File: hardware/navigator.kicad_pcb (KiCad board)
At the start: 4 copper layers, 65 x 56.5 mm, 45 parts, among them J1 BLDC-1, J10 GPIO, J2 BLDC-1, J3 BLDC-1, J4 BLDC-1, J5 BLDC-1, J6 BLDC-1, J7 Conn_01x02_Pin, J8 USB_C_Receptacle_USB2.0_16P, J9 Conn_01x04_Pin, SW1 SW_SPST, SW2 SW_SPST, U1 AP2112K-3.3, U2 LM2576-5.0, U3 ESP32-S3-MINI-1U, U4 INA226

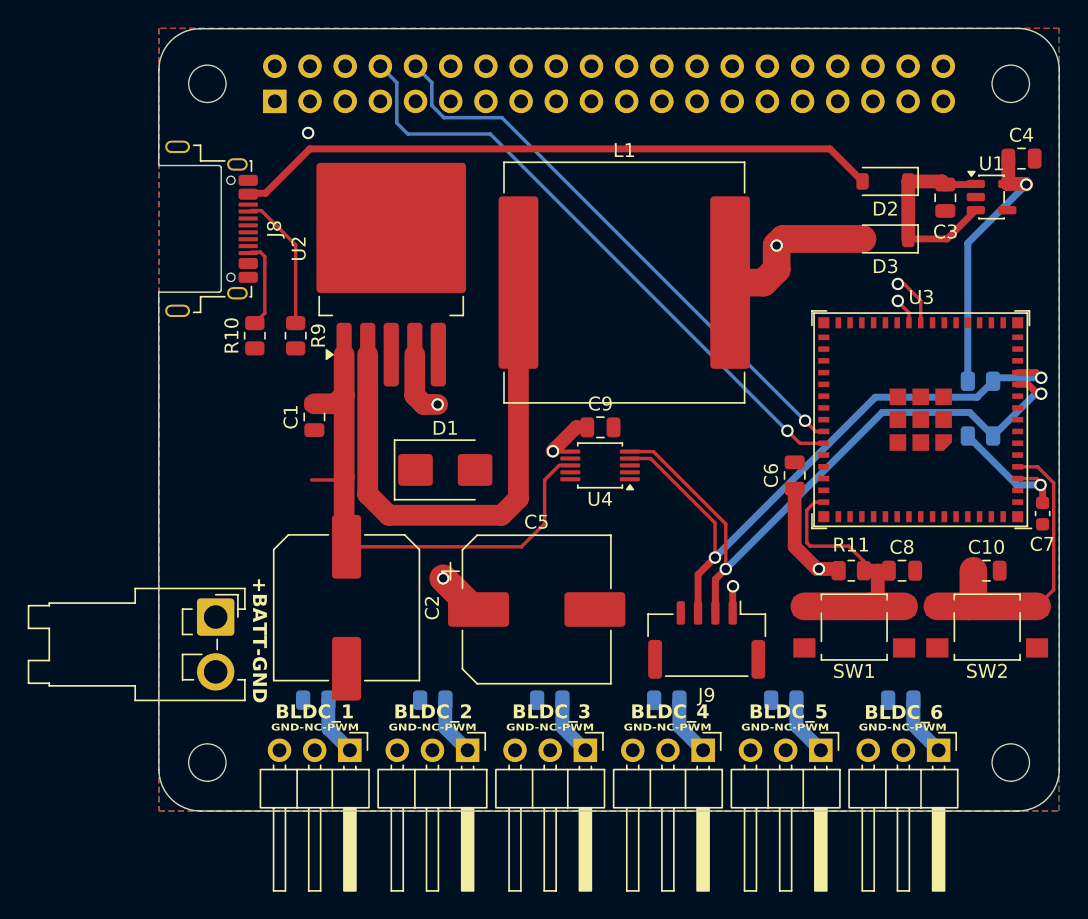
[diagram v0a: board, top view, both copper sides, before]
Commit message: feat: update navigator hardware to revision 002
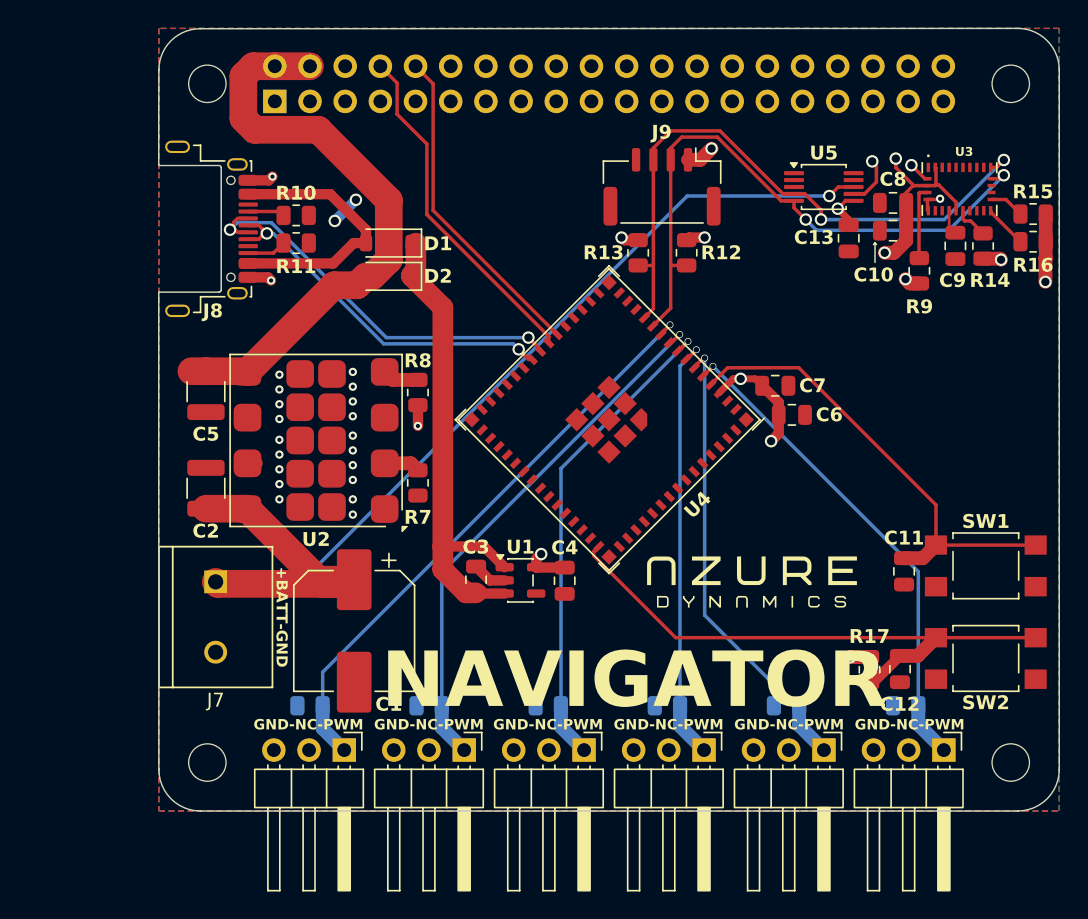
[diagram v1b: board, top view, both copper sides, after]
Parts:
- removed D3: D_Schottky, Diode_SMD:D_SOD-123
- removed L1: 100uH, Inductor_SMD:L_Vishay_IHLP-6767
- removed the U4 at (131.8, 75.0)
- added C11: 0.1uF, Capacitor_SMD:C_0805_2012Metric, F.Cu at (153.8, 82.7)
- added C12: 1uF, Capacitor_SMD:C_0805_2012Metric, F.Cu at (153.5, 89.8)
- added C13: 0.1uF, Capacitor_SMD:C_0805_2012Metric, F.Cu at (149.8, 58.6)
- added G***: LOGO, logo:logo, F.Cu at (142.8, 83.4)
- added R12: 2k2, Resistor_SMD:R_0805_2012Metric, F.Cu at (138.1, 59.7)
- added R13: 2k2, Resistor_SMD:R_0805_2012Metric, F.Cu at (134.6, 59.7)
- added R14: 10k, Resistor_SMD:R_0805_2012Metric, F.Cu at (159.5, 59.2)
- added R15: 10k, Resistor_SMD:R_0805_2012Metric, F.Cu at (163.1, 56.9)
- added R16: 10k, Resistor_SMD:R_0805_2012Metric, F.Cu at (163.1, 58.9)
- added R17: 10k, Resistor_SMD:R_0805_2012Metric, F.Cu at (151.3, 89.8)
- added U3: BNO086, BNO086:BNO086, F.Cu at (157.8, 55.1)
- added U5: INA226, Package_SO:TSSOP-10_3x3mm_P0.5mm, F.Cu at (148.0, 55.0)
- C1: value 0.1uF -> 100uF; footprint Capacitor_SMD:C_0805_2012Metric -> Capacitor_SMD:CP_Elec_8x10.5
- C2: value 330uF -> 10uF; footprint Capacitor_SMD:C_Elec_10x10.2 -> Capacitor_SMD:C_1210_3225Metric
- C5: value 1000uF -> 47uF; footprint Capacitor_SMD:CP_Elec_10x10.5 -> Capacitor_SMD:C_1210_3225Metric
- C7: footprint Capacitor_SMD:C_0603_1608Metric -> Capacitor_SMD:C_0805_2012Metric
- C8: value 1uF -> 0.1uF
- D1: value Schottky -> D_Schottky; footprint Diode_SMD:D_SMB -> Diode_SMD:D_SOD-123
- J7: footprint Connector_JST:JST_VH_S2P-VH_1x02_P3.96mm_Horizontal -> 282837-2:282837-2
- R11: value 10k -> 5k1
- R7: value 2k2 -> 100k; moved to F.Cu
- R8: value 2k2 -> 14k3; moved to F.Cu
- R9: value 5k1 -> 10k
- U2: value LM2576-5.0 -> MPM3550EGLE; footprint Package_TO_SOT_SMD:TO-263-5_TabPin3 -> Package_LGA:MPS_LGA-18-10EP_12x12mm_P3.3mm
- moved R11 46.5 mm to (109.9, 59.0), turned to 180 degrees
- moved R9 45.3 mm to (154.9, 61.0), turned to 90 degrees
- moved C4 44.9 mm to (129.3, 83.4), turned to -90 degrees
- moved U1 43.8 mm to (126.1, 83.3)
- moved C3 43.7 mm to (122.9, 83.3), turned to 90 degrees
- moved J6 42.9 mm to (113.4, 95.6)
- moved J1 42.9 mm to (156.7, 95.6)
- moved R6 42.7 mm to (110.9, 92.4)
- moved R1 42.6 mm to (153.9, 92.4)
- moved R7 40.8 mm to (118.7, 76.3), turned to 90 degrees
- moved R8 40.6 mm to (118.7, 69.8), turned to -90 degrees
- moved D2 36.5 mm to (116.6, 61.4)
- moved J9 32.9 mm to (136.3, 54.9)
- moved C9 28.8 mm to (157.5, 59.2), turned to -90 degrees
- moved C5 28.6 mm to (103.4, 69.7), turned to -90 degrees
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- renumbered U3 to U4
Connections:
- C1 pad 1: GND -> +BATT
- C1 pad 2: +BATT -> GND
- C10 pad 1: /BOOT -> +3V3
- C2 pad 1: +BATT -> GND
- C2 pad 2: GND -> +BATT
- C8 pad 1: /RST -> +3V3
- C9 pad 1: +3V3 -> Net-(U3-CAP)
- D1 pad 1: Net-(D1-K) -> +5V
- D1 pad 2: GND -> /USB_5V
- D2 pad 2: /USB_5V -> /BUCK_5V
- J1 pad 3: Net-(J1-Pin_3) -> GND
- R1 pad 2: Net-(J1-Pin_3) -> GND
- R10 pad 1: GND -> Net-(J8-CC1)
- R10 pad 2: Net-(J8-CC2) -> GND
- R11 pad 1: +3V3 -> GND
- R11 pad 2: /RST -> Net-(J8-CC2)
- R7 pad 1: +3V3 -> GND
- R7 pad 2: /I2C_SCL -> Net-(U2-RFREQ)
- R8 pad 1: +3V3 -> Net-(U2-FB)
- R8 pad 2: /I2C_SDA -> GND
- R9 pad 1: Net-(J8-CC1) -> +3V3
- R9 pad 2: GND -> Net-(U3-~{BOOT})
- SW1 pad 2: /RST -> /BOOT
- SW2 pad 2: /BOOT -> /RST
- U2 pad 1: +BATT -> unconnected-(U2-EN-Pad1)
- U2 pad 2: Net-(D1-K) -> Net-(U2-RFREQ)
- U2 pad 3: GND -> unconnected-(U2-PGOOD-Pad3)
- U2 pad 4: /BUCK_5V -> Net-(U2-FB)
- U2 pad 5: GND -> /BUCK_5V
- U4 pad 21: unconnected-(U3-IO17-Pad21) -> /GPIO15/RXD0
- U4 pad 22: unconnected-(U3-IO18-Pad22) -> /GPIO14/TXD0
- U4 pad 39: /GPIO15/RXD0 -> unconnected-(U4-TXD0-Pad39)
- U4 pad 40: /GPIO14/TXD0 -> unconnected-(U4-RXD0-Pad40)
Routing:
- net +BATT: track 39.2 -> 80.8 mm, vias 0 -> 1
- net /BLDC_6: track 4.37 -> 42.7 mm, vias 0 -> 1
- net Net-(D1-K): track 37.7 -> 0.00 mm
- net /BLDC_5: track 4.35 -> 38.8 mm, vias 0 -> 1
- net /BLDC_1: track 4.26 -> 35.8 mm, vias 0 -> 1
- net /BLDC_4: track 4.32 -> 35.0 mm, vias 0 -> 1
- net /BLDC_2: track 4.28 -> 33.1 mm, vias 0 -> 1
- net /USB_5V: track 46.5 -> 19.6 mm
- net /BLDC_3: track 4.30 -> 31.1 mm, vias 0 -> 1
- net /USB_D-: track 3.67 -> 29.8 mm, vias 1 -> 2
- net /USB_D+: track 1.91 -> 26.0 mm, vias 1 -> 2
- net /RST: track 21.0 -> 41.3 mm
- net +5V: track 14.9 -> 34.9 mm
- net /GPIO14/TXD0: track 45.0 -> 25.0 mm, vias 1 -> 0
- net /GPIO15/RXD0: track 41.4 -> 23.6 mm, vias 1 -> 0
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- removed copper zone on In2.Cu, net /BUCK_5V
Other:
- board text added: "01 --> BLDC_1 02 --> BLDC_2 03 --> BLDC_3 04 --> BLDC_4 05 --> BLDC_5 06 --> BLDC_6 07 --> I2C_SCL 08 <-> I2C_SDA 17 --> UART_TX 18 <-- UART_RX"
- board text added: "Designed by alexs (getriscvyy)"
- board text added: "NAVIGATOR"
- board text added: "{ "ViaStitcher": "0.3.1", "stitch_zone_0": { "HSpacing": "1", "VSpacing": "1", "HOffset": "0", "VOffset": "0", "Clearance": "0", "Randomize": false, "Stagger": true, "OnlyFilledCopper": true }, "stitch_zone_1": { "HSpacing": "5", "VSpacing": "5", "HOffset": "0", "VOffset": "0", "Clearance": "0.5", "Randomize": false, "Stagger": false, "OnlyFilledCopper": true } }"
- board text removed: "BLDC_1"
- board text removed: "BLDC_2"
- board text removed: "BLDC_3"
- board text removed: "BLDC_4"
- board text removed: "BLDC_5"
- board text removed: "BLDC_6"
